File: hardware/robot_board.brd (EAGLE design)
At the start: 95.2 x 76.1 mm, 135 parts, among them J1 POWER_JACKPTH, Q1 DMP2035U, Q2 DMP2035U, Q3 DMP2035U-7, Q4 DMP2035U-7, U1 FT232RL-BASICSSOP, U11 LM393, U12 LM393, U16 LM393, U17 ATMEGA325PA, U2 SIA907EDJT, U3 MIC5219, U5 SIA907EDJT, U6 SIA907EDJT, U7 TLV70233, Y1 16MHz

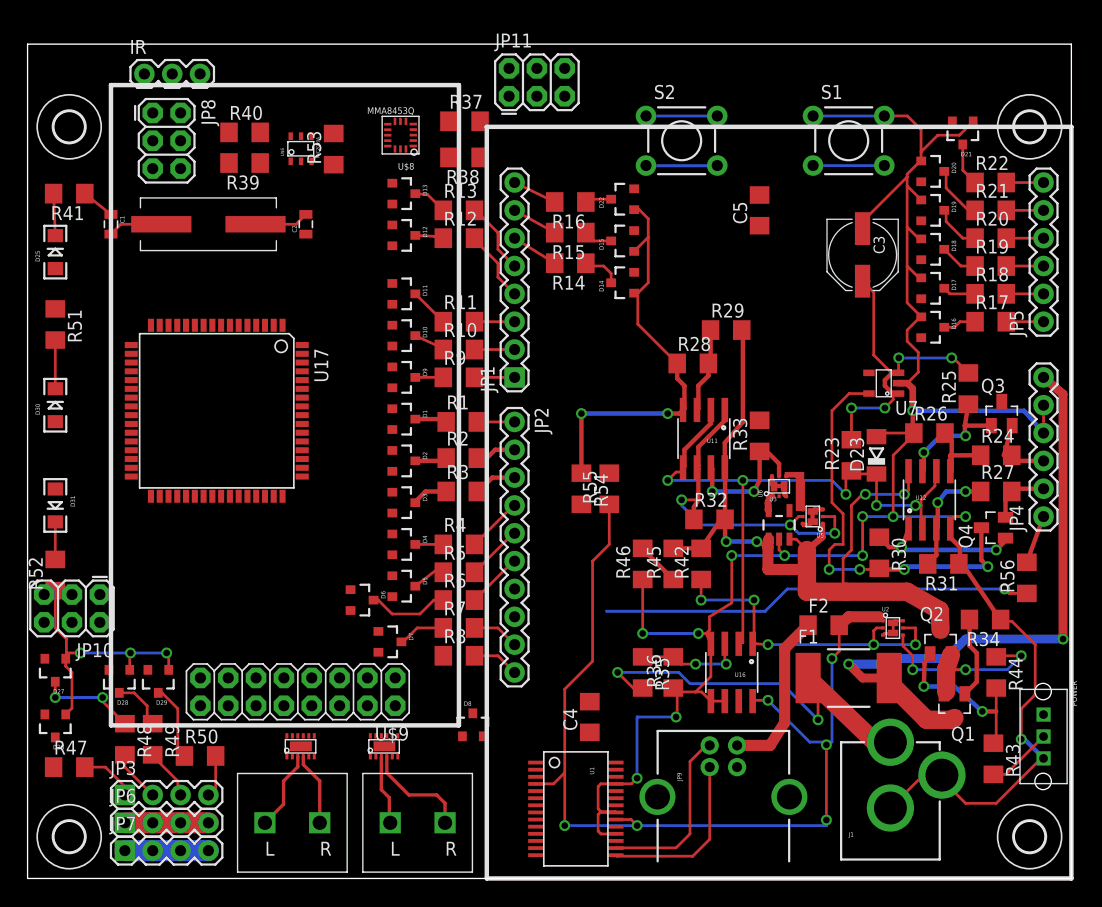
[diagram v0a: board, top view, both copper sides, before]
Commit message: more routing
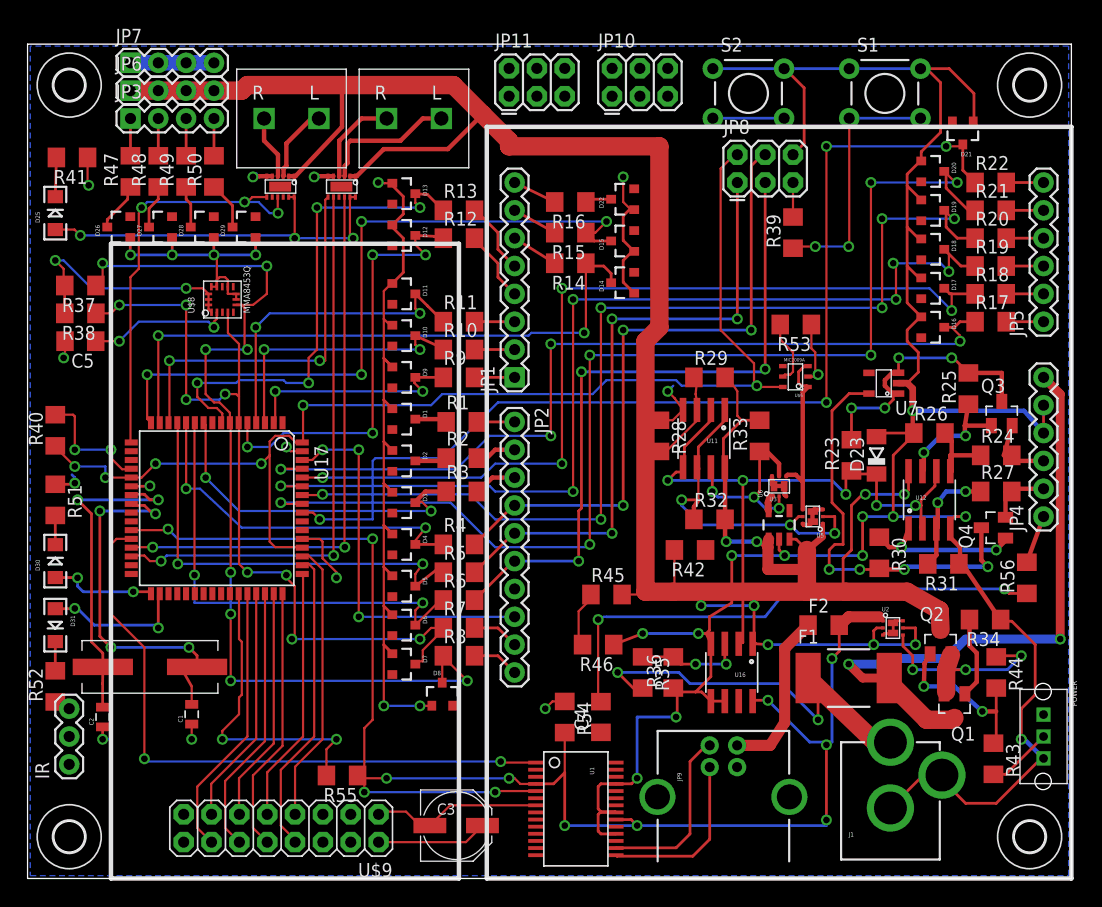
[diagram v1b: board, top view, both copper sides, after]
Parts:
- moved JP7 71.9 mm to (9.40, 74.4)
- moved JP6 66.8 mm to (9.40, 71.9)
- moved JP10 65.2 mm to (53.3, 71.4), turned to 0 degrees
- moved U$19 64.5 mm to (32.8, 69.3), turned to 180 degrees
- moved U$20 64.5 mm to (21.6, 69.3), turned to 180 degrees
- moved C3 63.9 mm to (39.1, 4.83), turned to 0 degrees
- moved IR 63.4 mm to (3.81, 10.4), turned to 90 degrees
- moved C5 63.1 mm to (4.83, 49.0), turned to 180 degrees
- moved JP3 61.7 mm to (9.40, 69.3)
- moved R47 54.6 mm to (9.40, 64.5), turned to 90 degrees
- moved JP8 53.7 mm to (64.8, 63.5), turned to 0 degrees
- moved R50 53.4 mm to (17.0, 64.5), turned to 90 degrees
- moved U$4 52.4 mm to (29.5, 63.8), turned to 180 degrees
- moved U$5 52.3 mm to (23.9, 63.8), turned to 180 degrees
- moved R48 51.9 mm to (11.9, 64.5), turned to 90 degrees
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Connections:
- net 5V: no longer JP6.1, JP6.2, JP6.3, JP6.4
- net VIN_F: now also JP6.1, JP6.2, JP6.3, JP6.4
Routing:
- net VIN_F: track 77.0 -> 206.8 mm
- net GND: track 293.7 -> 408.7 mm, vias 17 -> 33
- net 5V_UC: track 0.00 -> 109.7 mm, vias 0 -> 6
- net A4_IN: track 5.08 -> 105.2 mm, vias 0 -> 6
- net A5_IN: track 3.94 -> 95.4 mm, vias 0 -> 4
- net SDA_IN: track 0.00 -> 90.4 mm, vias 0 -> 8
- net A3_IN: track 4.36 -> 93.8 mm, vias 0 -> 6
- net A2_IN: track 3.44 -> 90.3 mm, vias 0 -> 6
- net A1_IN: track 3.02 -> 81.2 mm, vias 0 -> 4
- net A0_IN: track 3.02 -> 78.3 mm, vias 0 -> 4
- net SCL_IN: track 4.35 -> 75.6 mm, vias 0 -> 8
- net D6_IN: track 2.62 -> 65.3 mm, vias 0 -> 4
- net TX: track 0.00 -> 61.7 mm, vias 0 -> 4
- net RX: track 0.00 -> 58.7 mm, vias 0 -> 2
- net D13: track 5.13 -> 62.2 mm, vias 0 -> 3
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- added copper zone on layer 16, net GND

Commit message: more routing
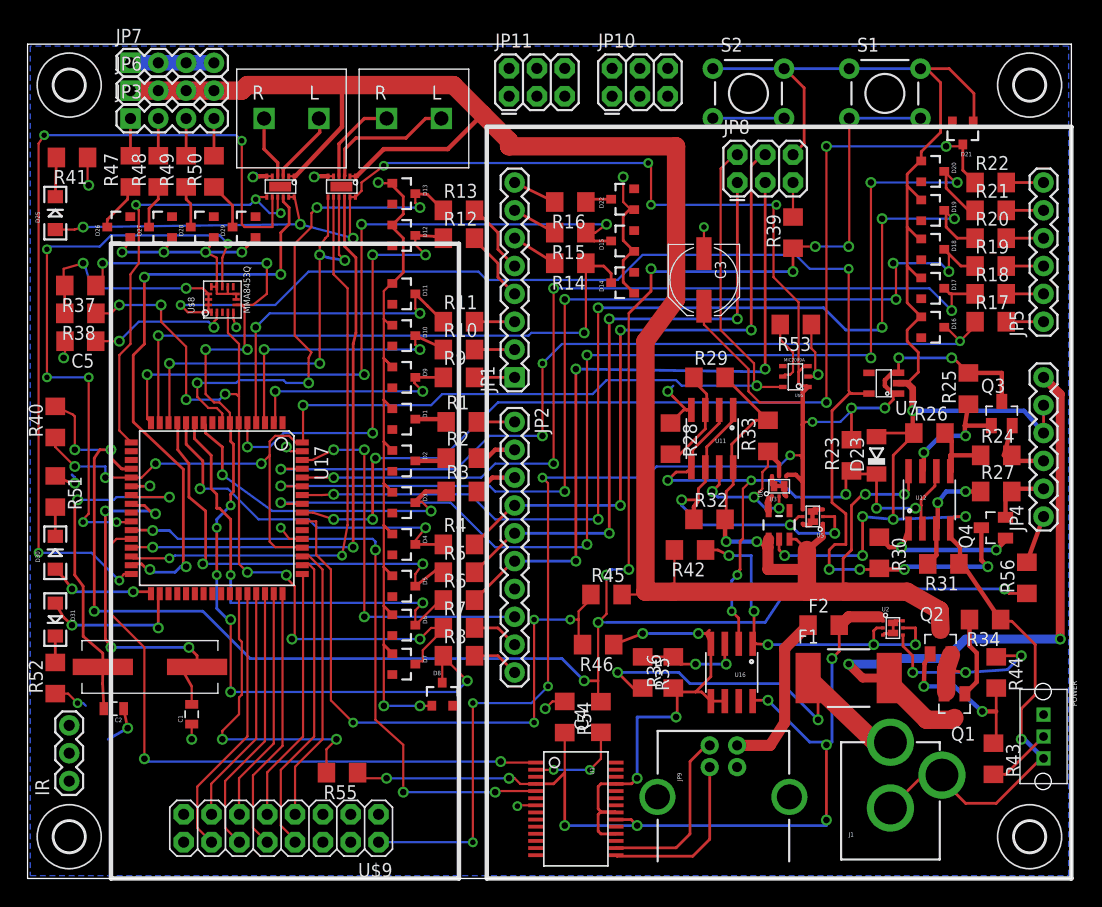
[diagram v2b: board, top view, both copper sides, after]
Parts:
- moved C3 54.7 mm to (61.7, 54.6), turned to 270 degrees
- moved IR 1.52 mm to (3.81, 8.89)
- moved C2 1.27 mm to (7.87, 15.5), turned to 180 degrees
- moved R28 1.05 mm to (58.7, 40.1)
- moved D30 0.76 mm to (2.54, 29.7)
- moved R40 0.76 mm to (2.54, 41.7)
- moved R51 0.76 mm to (2.54, 35.3)
- moved R52 0.76 mm to (2.54, 18.3)
- moved U11 0.76 mm to (62.5, 40.1)
- moved R33 0.76 mm to (67.6, 40.4)
- moved D31 0.51 mm to (2.54, 23.6)
- moved R55 0.25 mm to (28.7, 9.65)
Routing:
- net 5V: track 87.7 -> 229.0 mm, vias 7 -> 17
- net RESET: track 82.8 -> 200.1 mm, vias 6 -> 12
- net M1_DIR1: track 0.00 -> 79.6 mm, vias 0 -> 4
- net 3V3: track 63.1 -> 141.0 mm, vias 6 -> 8
- net ACCEL_INT: track 0.00 -> 54.7 mm, vias 0 -> 6
- net M1_DIR0: track 0.00 -> 54.6 mm, vias 0 -> 4
- net N$52: track 5.18 -> 56.2 mm, vias 0 -> 4
- net GND: track 408.7 -> 390.8 mm, vias 33 -> 36
- net DTR: track 0.00 -> 8.78 mm, vias 0 -> 2
- net M0_EN: track 34.9 -> 43.0 mm, vias 2 -> 4
- net USBGATE: track 28.1 -> 32.2 mm
- net SDA_IN: track 90.4 -> 93.4 mm, vias 8 -> 10
- net TX: track 61.7 -> 58.8 mm
- net A3_IN: track 93.8 -> 96.5 mm
- net N$3: track 29.9 -> 32.5 mm
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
